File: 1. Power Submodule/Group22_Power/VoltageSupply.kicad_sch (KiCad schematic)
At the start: 41 parts, among them J3 USB_Micro_B_Female_Connector, J8 USB_C_Receptacle, Q1 Si2301CDS, U1 TPS61093, U2 HT75xx-1-SOT89, U4 TP4056_1

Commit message: power:
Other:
- moved on the sheet: BT1, BT2, C1, C2, C3, C4, C5, C6, C7, C8, C9, D2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

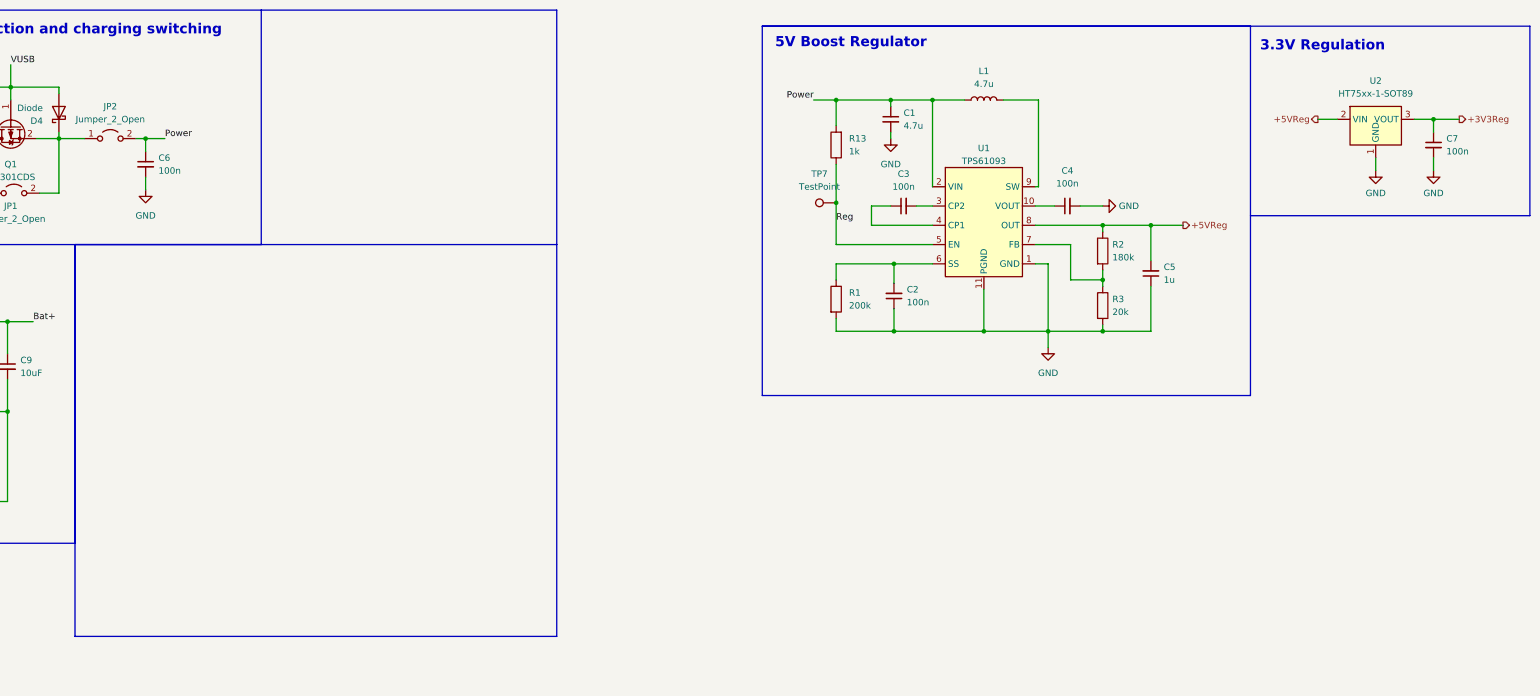
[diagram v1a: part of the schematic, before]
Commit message: $1
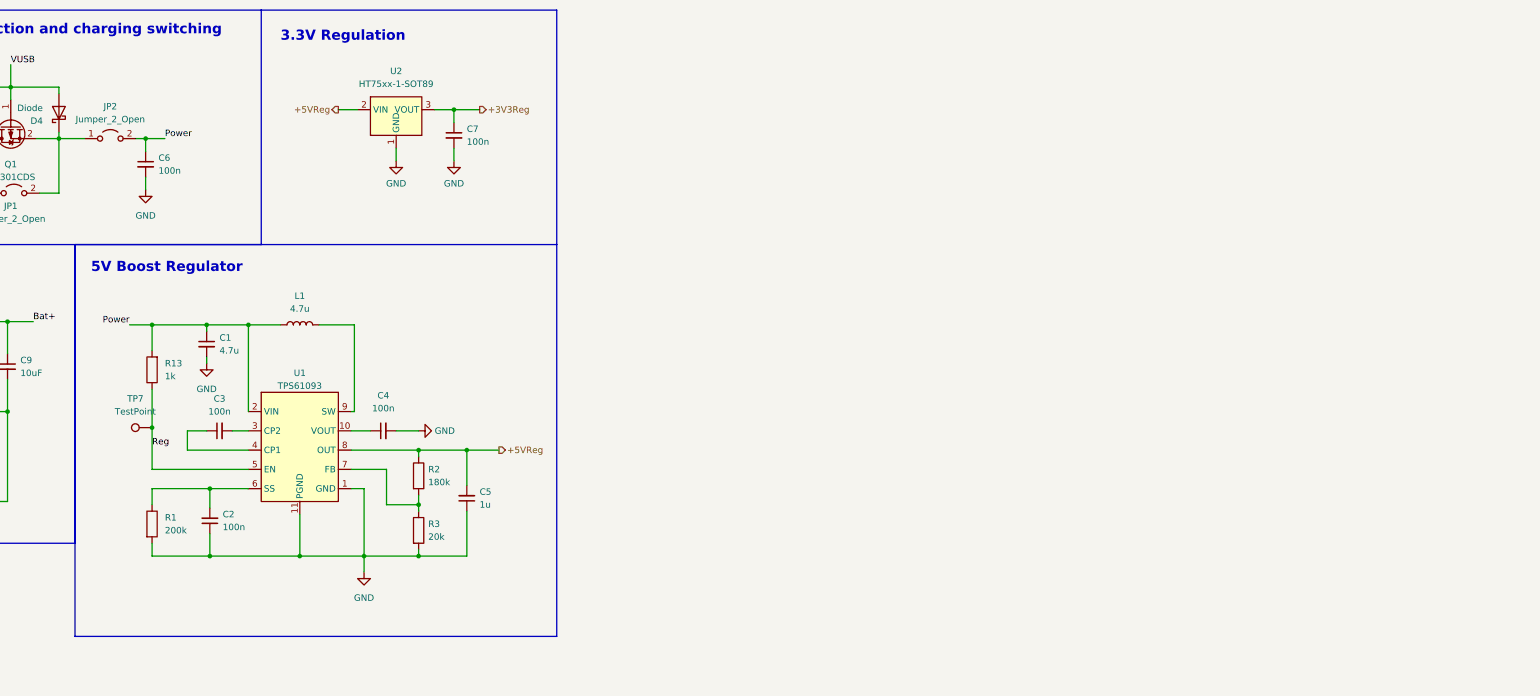
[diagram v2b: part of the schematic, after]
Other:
- moved on the sheet: C1, C2, C3, C4, C5, C7, L1, R1, R13, R2, R3, TP7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
